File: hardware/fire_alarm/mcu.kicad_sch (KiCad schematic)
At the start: 23 parts, among them J2 USB_C_Receptacle_USB2.0_16P, Q1 MMBT3904 40V 0.2A, Q2 MMBT3904 40V 0.2A, SW1 SW_Push, SW2 SW_Push, U3 CH340C, U4 ESP32-WROOM-32

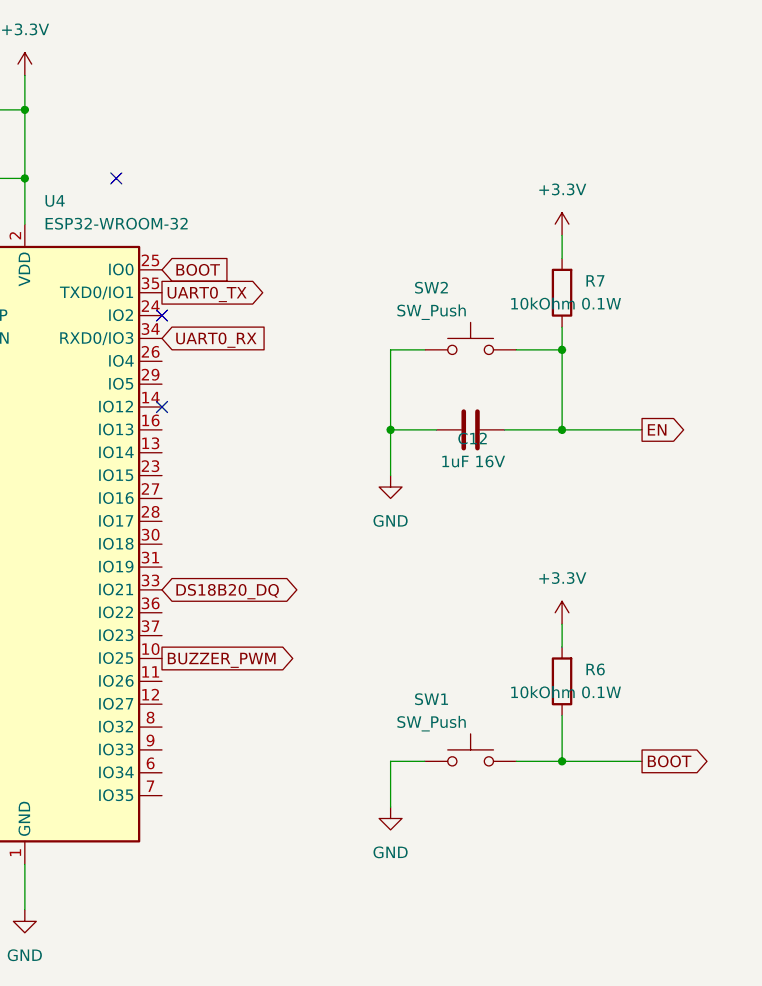
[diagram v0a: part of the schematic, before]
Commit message: feat: complete schematic
Signed-off-by: Trung Hieu Nguyen <hieu.nguyenarc03@gmail.com>
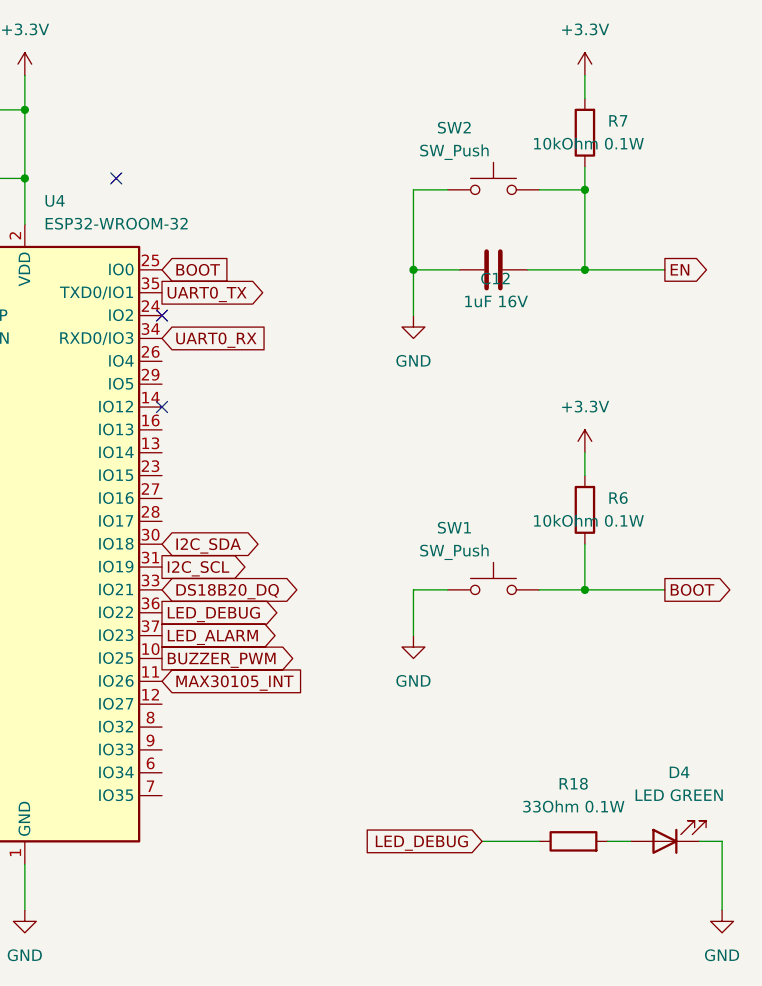
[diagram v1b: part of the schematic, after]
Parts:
- added D4: LED GREEN, LED_SMD:LED_0805_2012Metric_Pad1.15x1.40mm_HandSolder, symbol Device:LED
- added R18: 33Ohm 0.1W, Resistor_SMD:R_0603_1608Metric_Pad0.98x0.95mm_HandSolder, symbol Device:R
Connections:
- net GND: now also D4.1 (K)
- net MAX30105_INT: now reaches U4.11 (IO26)
- net I2C_SDA: now reaches U4.30 (IO18)
- net I2C_SCL: now reaches U4.31 (IO19)
- net LED_DEBUG: now reaches U4.36 (IO22)
- net LED_DEBUG: now also R18.1
- net LED_ALARM: now reaches U4.37 (IO23)
- new net: D4.2 (A), R18.2
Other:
- moved on the sheet: C12, R6, R7, SW1, SW2
